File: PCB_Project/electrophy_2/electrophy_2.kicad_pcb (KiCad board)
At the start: 4 copper layers, 35 x 35 mm, 46 parts, among them IC1 ESP32-C3FN4, J1 USB_C_Receptacle_USB2.0_14P, J3 Conn_01x04, SW2 SW_Push, U1 LSM6DSV320XTR, U2 BQ21040DBV, U3 TPS27081ADDCR, U4 USBLC6-2SC6, U5 MIC5504-3.3YM5, Y1 40MHZ 15pf, Y2 32 KHz

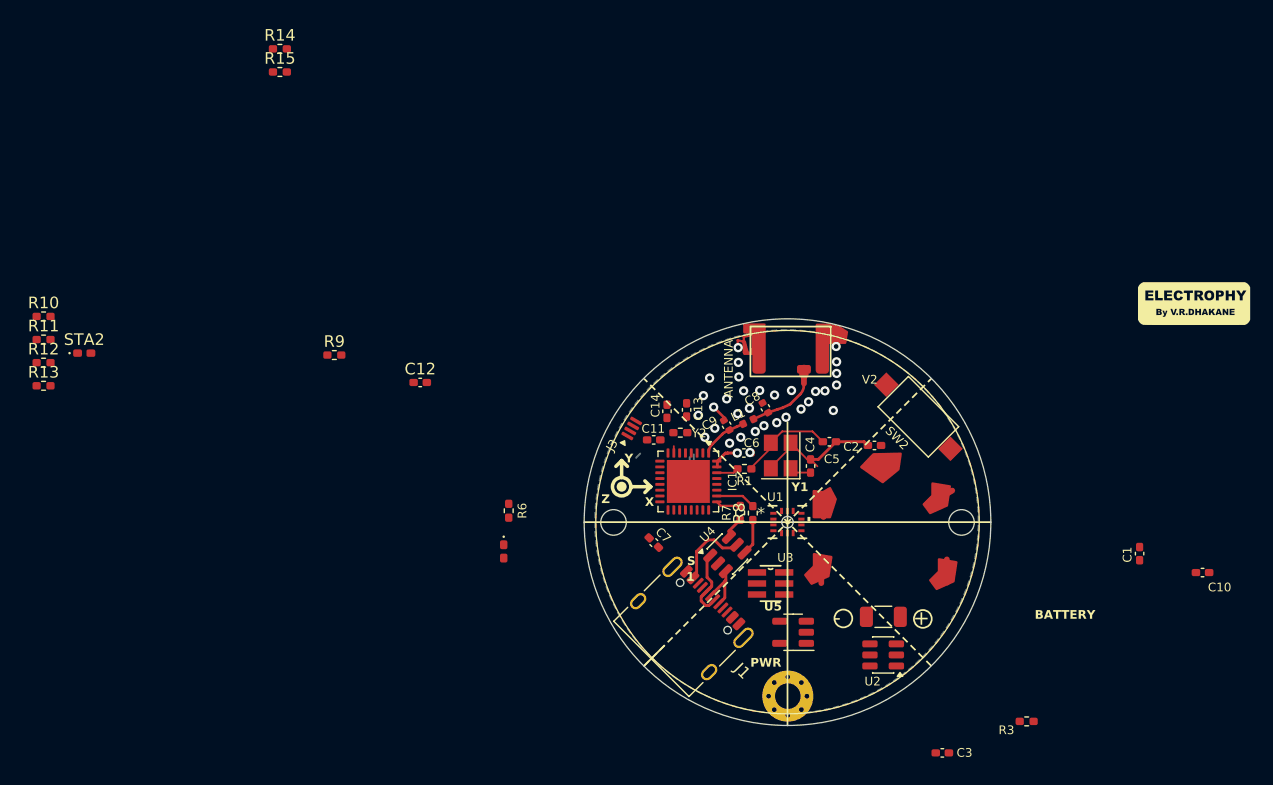
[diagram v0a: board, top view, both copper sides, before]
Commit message: PCB draft
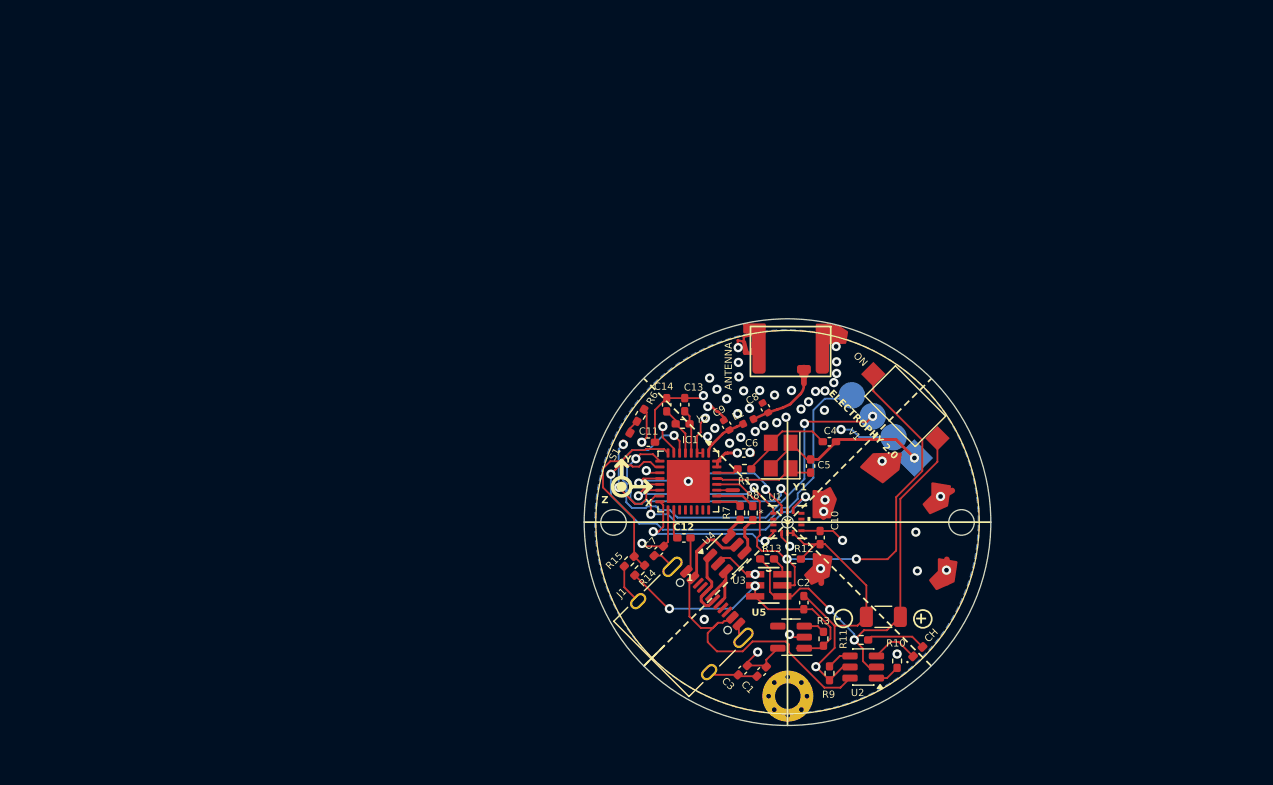
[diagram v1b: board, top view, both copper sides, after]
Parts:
- removed G***: LOGO, ESP32 IMU:Electrophy logo
- J3: footprint Connector_FFC-FPC:Amphenol_F32R-1A7x1-11004_1x04-1MP_P0.5mm_Horizontal -> pogo_pads_4:pogo_pads_4; moved to B.Cu
- moved R10 79.2 mm to (159.5, 112.0), turned to 90 degrees
- moved CH 76.2 mm to (161.2, 111.2), turned to 45 degrees
- moved R11 75.0 mm to (156.4, 110.2)
- moved R12 66.8 mm to (150.6, 103.2)
- moved R13 64.0 mm to (148.3, 103.2)
- moved R14 54.5 mm to (137.3, 104.2), turned to 45 degrees
- moved R15 51.7 mm to (136.4, 103.4), turned to -135 degrees
- moved R9 50.7 mm to (153.6, 113.1), turned to -90 degrees
- moved C1 34.1 mm to (147.8, 112.9), turned to -135 degrees
- moved C10 33.1 mm to (152.8, 101.4), turned to -90 degrees
- moved C12 26.3 mm to (141.1, 101.4)
- moved J3 23.0 mm to (159.6, 90.5), turned to 135 degrees
- moved R3 18.9 mm to (153.1, 110.1), turned to 90 degrees
- moved C3 18.6 mm to (146.2, 112.8), turned to -135 degrees
- moved C2 14.8 mm to (151.4, 107.0), turned to 90 degrees
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- renumbered STA2 to CH, SW2 to ON, STA1 to S1
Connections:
- BAT1 pad 1: BAT_V -> Net-(BAT1-Pin_1)
- C2 pad 1: Net-(U5-VIN) -> BAT_V
- J3 pad 3: SDA -> SCL
- J3 pad 4: SCL -> SDA
- ON pad 1: BAT_V -> Net-(BAT1-Pin_1)
- R11 pad 1: BAT_V -> Net-(BAT1-Pin_1)
- R13 pad 1: BAT_V -> Net-(BAT1-Pin_1)
- R3 pad 1: Net-(U5-VIN) -> BAT_V
- U2 pad 2: BAT_V -> Net-(BAT1-Pin_1)
- U3 pad 2: Net-(U5-VIN) -> BAT_V
- U3 pad 3: Net-(U5-VIN) -> BAT_V
- U3 pad 4: BAT_V -> Net-(BAT1-Pin_1)
- U5 pad 1: Net-(U5-VIN) -> BAT_V
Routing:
- net GND: track 23.5 -> 83.1 mm, vias 32 -> 41
- net POWER_HOLD: track 0.00 -> 42.4 mm, vias 0 -> 2
- net SCL: track 0.75 -> 39.1 mm, vias 0 -> 3
- net Net-(BAT1-Pin_1): track 0.00 -> 38.0 mm, vias 0 -> 2
- net +3.3V: track 3.07 -> 34.3 mm, vias 1 -> 10
- net SDA: track 0.00 -> 27.9 mm, vias 0 -> 1
- net CS: track 0.00 -> 27.6 mm, vias 0 -> 2
- net VBUS: track 6.68 -> 32.2 mm
- net BAT_V: track 0.00 -> 25.2 mm, vias 0 -> 2
- net SCLK: track 0.00 -> 22.6 mm, vias 0 -> 2
- net MOSI: track 0.00 -> 16.5 mm, vias 0 -> 2
- net BAT_MON: track 0.51 -> 16.3 mm
- net MISO: track 0.00 -> 15.5 mm, vias 0 -> 2
- net INT1: track 0.00 -> 14.5 mm, vias 0 -> 2
- net Net-(IC1-GPIO8): track 0.00 -> 8.82 mm, vias 0 -> 2
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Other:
- rule solder_mask_min_width: 0.125 -> 0.1524
- board text added: "3.3v"
- board text added: "ELECTROPHY 2.0"
- board text added: "GND"
- board text added: "SCL"
- board text added: "SDA"
- board text added: "V1"
- board text removed: "BATTERY"
- board text removed: "PWR"
- board text removed: "S"
- board text removed: "V2"
